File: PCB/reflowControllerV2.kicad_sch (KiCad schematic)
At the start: 96 parts, among them J10 NEXTION_OB, J11 PWR, J12 A-1JB, J2 SSR2, J3 SSR1, J4 FAN1, J5 FAN2, J6 T1, J7 T2, J8 SWD, J9 NEXTION_FRONT, Q1 BSS316NH6327, Q2 BSS316NH6327, Q3 BSS316NH6327, Q4 BSS316NH6327, Q5 BSS316NH6327, SW1 B3F-4055, U1 918-468K2029E50001, U10 ZD24C128A, U2 918-468K2029E50001, U3 AMS1117-3.3, U4 STM32WBxx_QFN48, U5 USBLC6-2SC6, U6 USBLC6-2SC6, U7 CH340G, U8 MAX31855KASA, U9 MAX31855KASA, Y1 NX2016_32MHz, Y2 NX2012_32K768Hz, Y3 12M

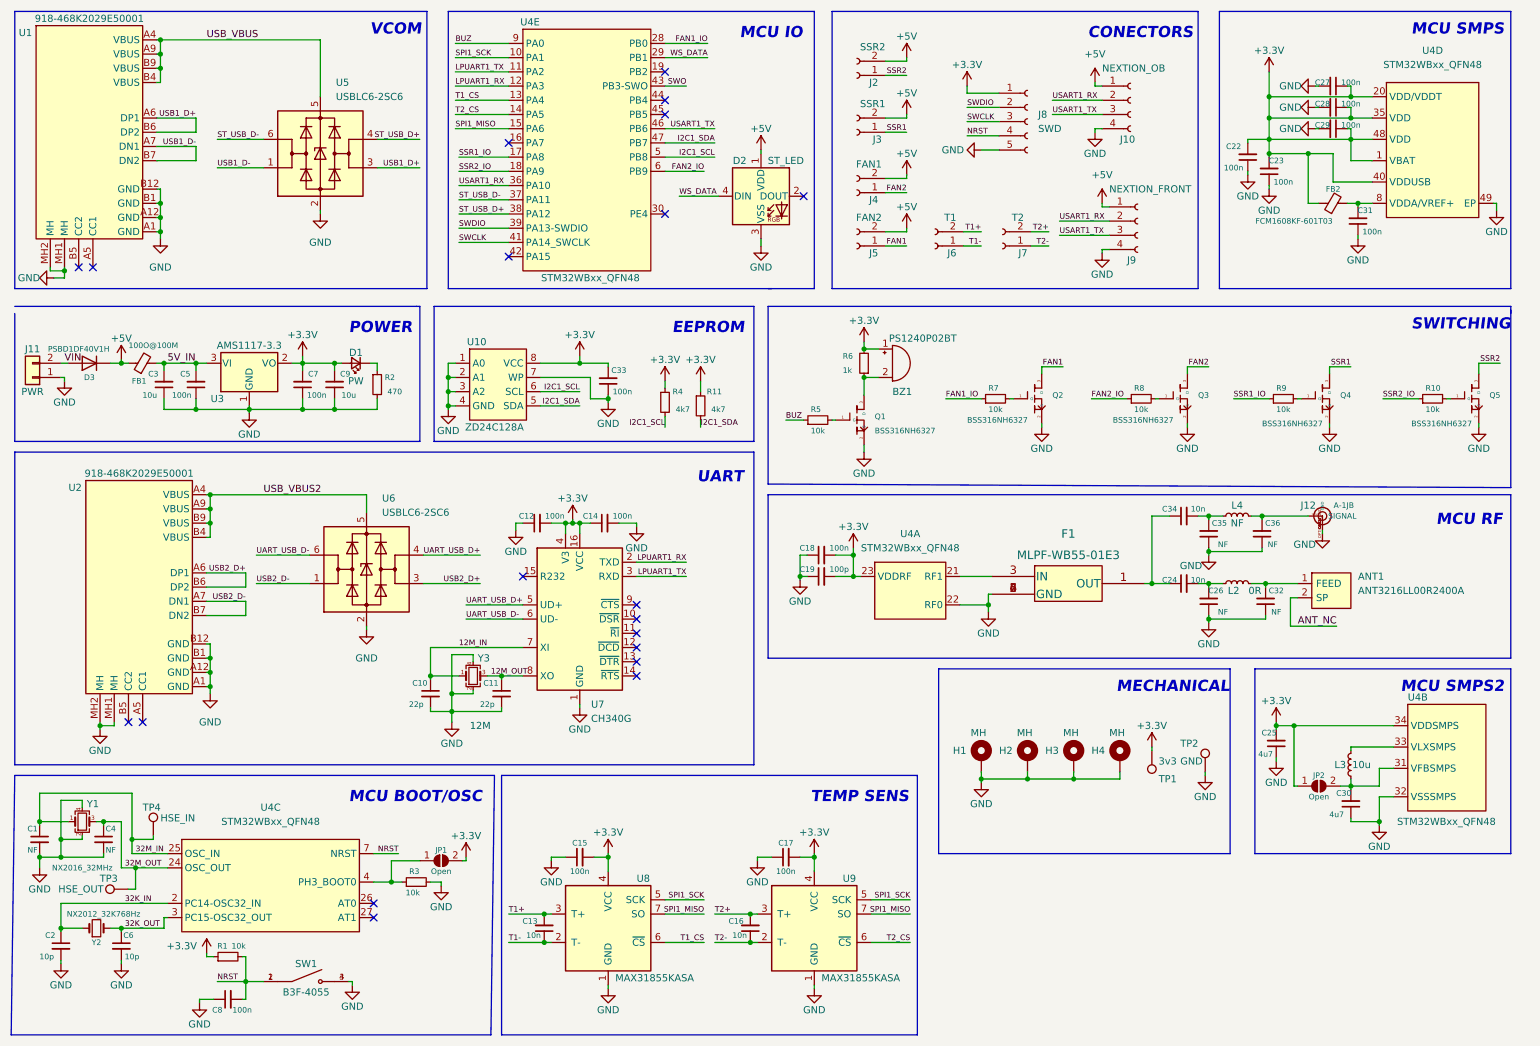
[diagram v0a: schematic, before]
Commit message: Few changes
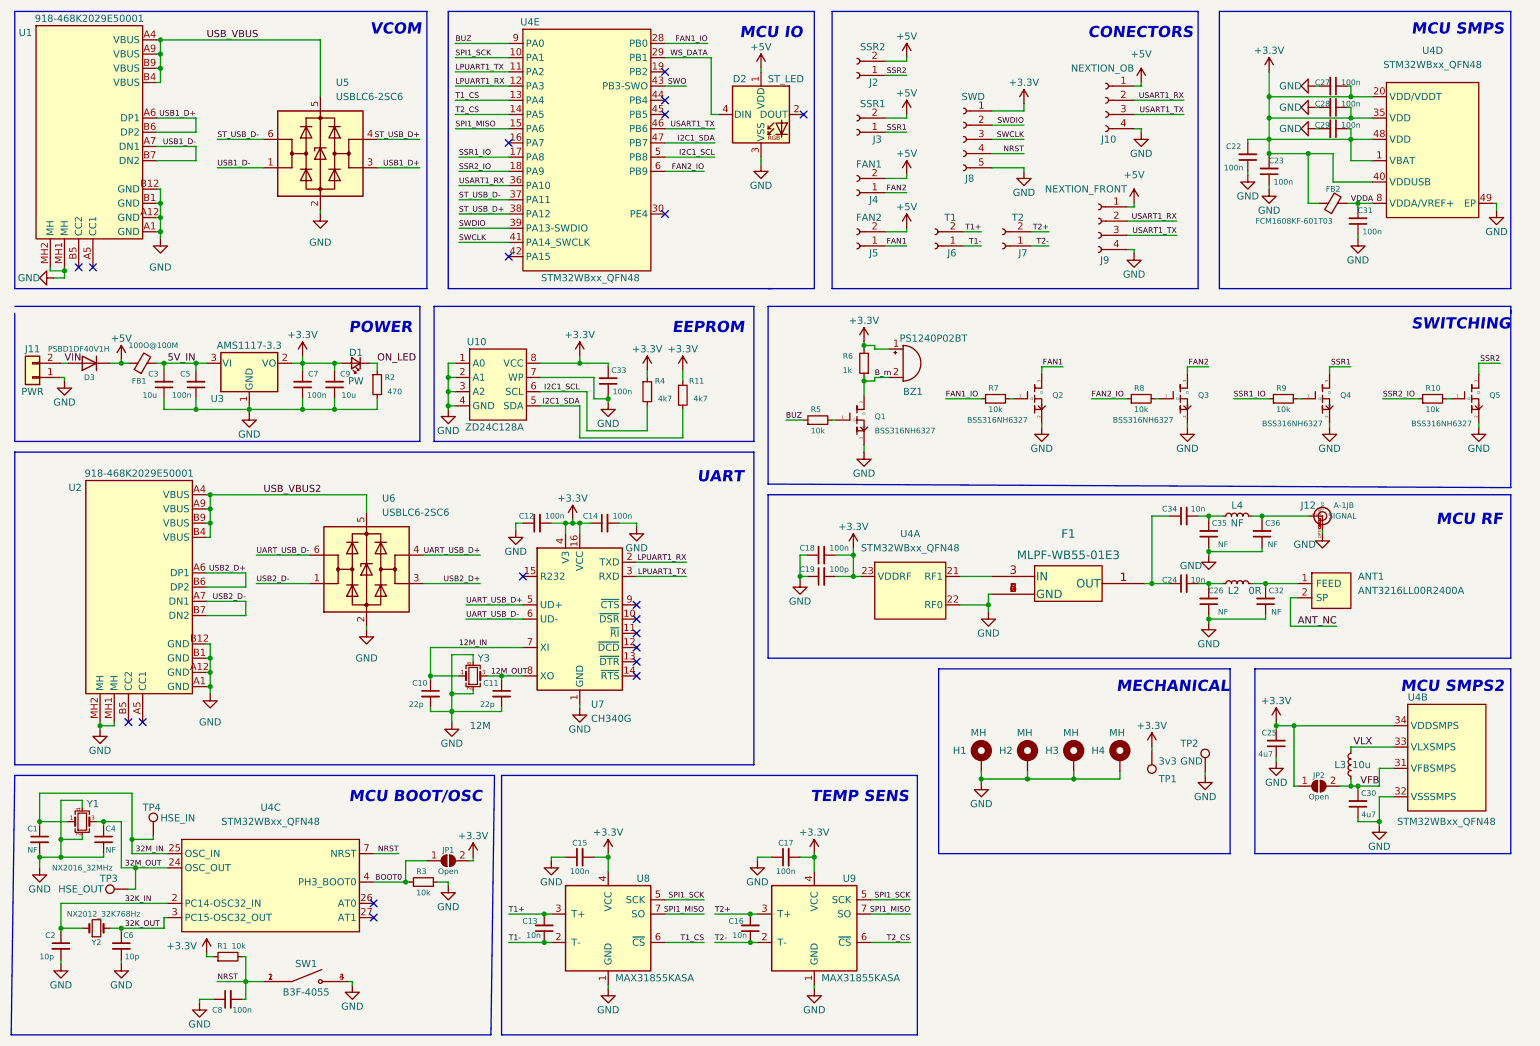
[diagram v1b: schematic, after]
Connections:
- net B_m: now reaches BZ1.2 (+), Q1.3 (D), R6.1
- net ON_LED: now reaches D1.1 (K), R2.1
- net VDDA: now reaches C31.2, FB2.2, U4.8 (VDDA/VREF+)
- net BOOT0: now reaches JP1.1 (A), R3.1, U4.4 (PH3_BOOT0)
- net VFB: now reaches C30.2, JP2.2 (B), L3.1, U4.31 (VFBSMPS)
- net VLX: now reaches L3.2, U4.33 (VLXSMPS)
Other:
- moved on the sheet: BZ1, C30, D2, J10, J8, J9, JP1, R11, R3, R4
